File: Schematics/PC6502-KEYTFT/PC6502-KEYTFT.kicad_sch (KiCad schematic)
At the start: 47 parts, among them J1 BUS, J2 Conn_02x20_Odd_Even, J5 Conn_02x05_Odd_Even, J6 MTJ-88ARX1-FSM-LG, Q7 2N3904, Q8 2N3904, U1 W65C51NxP, U2 ATF1502AS, U21 AMS1117-3.3, U8 TXB0108PW, U9 TXB0108PW, X2 1.8432MHz

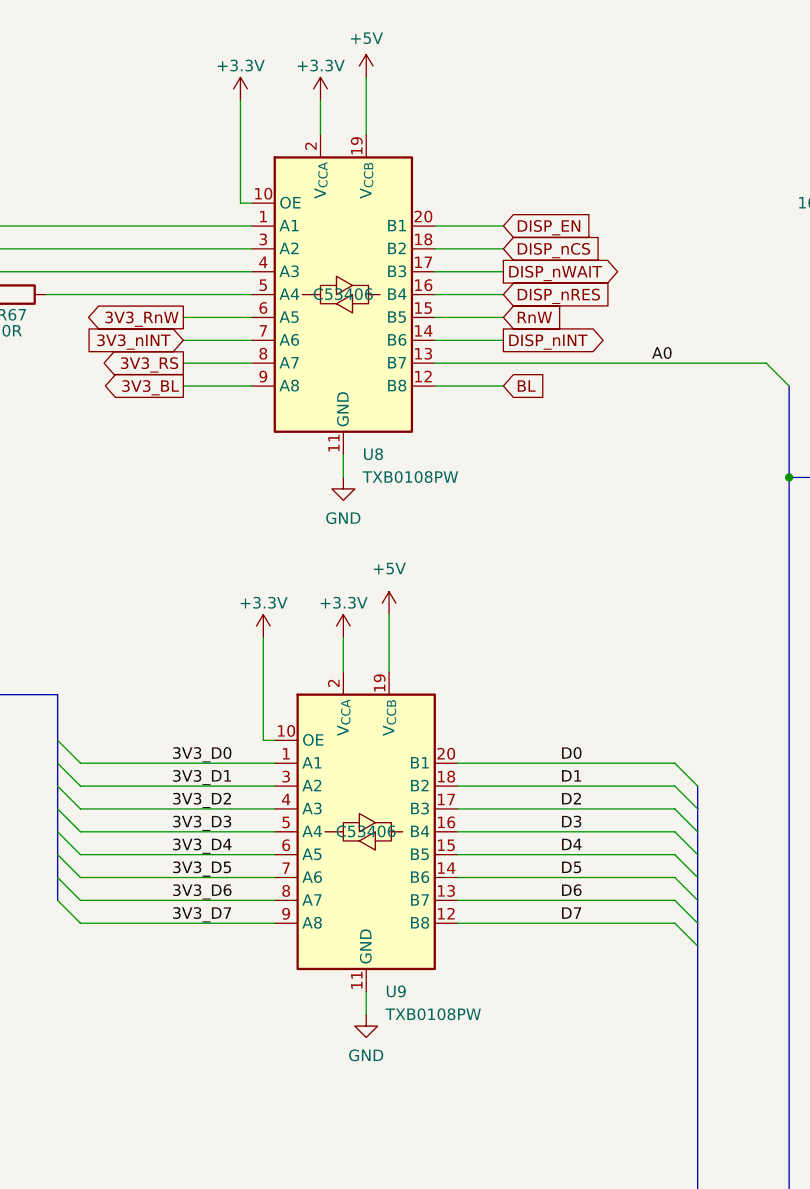
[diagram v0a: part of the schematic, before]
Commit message: Update KeyTFT CPLD
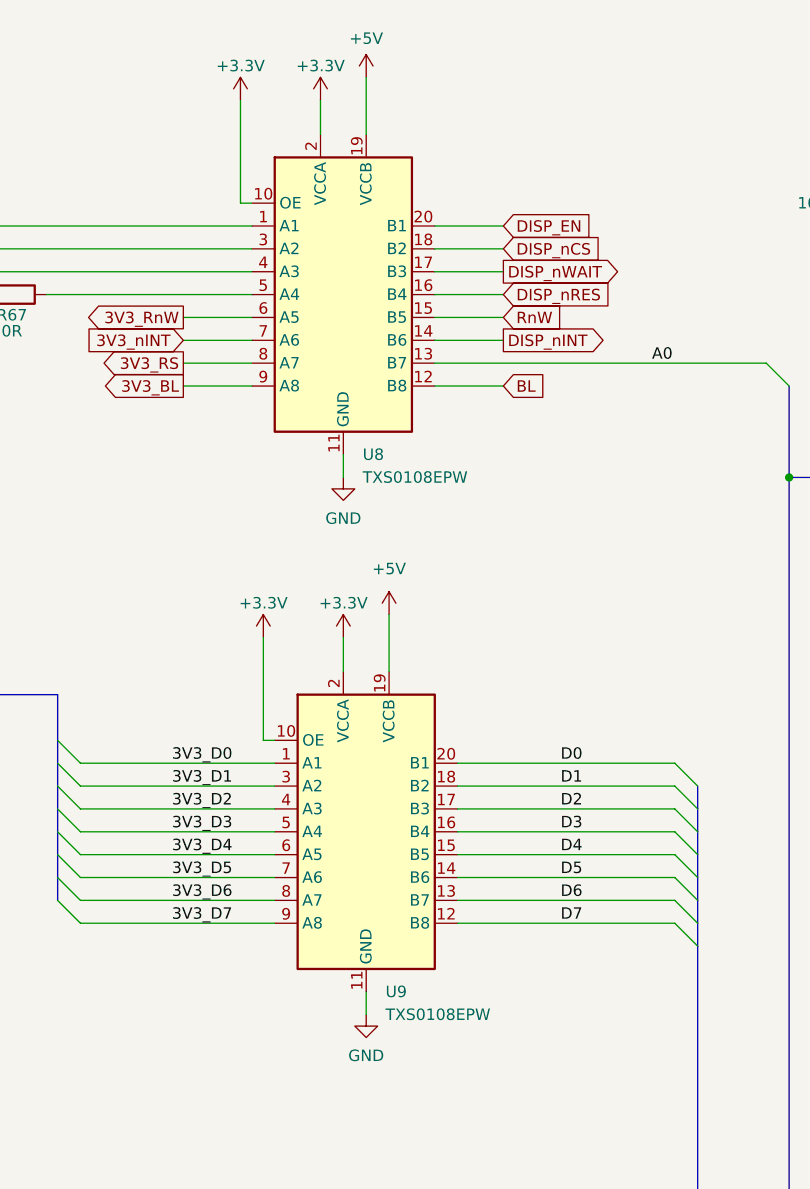
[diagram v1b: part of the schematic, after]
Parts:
- removed U8, U9: TXB0108PW, Package_SO:TSSOP-20_4.4x6.5mm_P0.65mm, symbol Logic_LevelTranslator:TXB0108PW
- added U8, U9: TXS0108EPW, Package_SO:TSSOP-20_4.4x6.5mm_P0.65mm, symbol Logic_LevelTranslator:TXS0108EPW
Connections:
- net +3.3V: now also U8.10 (OE), U8.2 (VCCA), U9.10 (OE), U9.2 (VCCA)
- net +5V: now also U8.19 (VCCB), U9.19 (VCCB)
- net 3V3_BL: now also U8.9 (A8)
- net 3V3_D0: now also U9.1 (A1)
- net 3V3_D1: now also U9.3 (A2)
- net 3V3_D2: now also U9.4 (A3)
- net 3V3_D3: now also U9.5 (A4)
- net 3V3_D4: now also U9.6 (A5)
- net 3V3_D5: now also U9.7 (A6)
- net 3V3_D6: now also U9.8 (A7)
- net 3V3_D7: now also U9.9 (A8)
- net 3V3_EN: now also U8.1 (A1)
- net 3V3_RS: now also U8.8 (A7)
- net 3V3_RnW: now also U8.6 (A5)
- net 3V3_nCS: now also U8.3 (A2)
- net 3V3_nINT: now also U8.7 (A6)
- net 3V3_nWAIT: now also U8.4 (A3)
- net A0: now also U8.13 (B7)
- net BL: now also U8.12 (B8)
- net D0: now also U9.20 (B1)
- net D1: now also U9.18 (B2)
- net D2: now also U9.17 (B3)
- net D3: now also U9.16 (B4)
- net D4: now also U9.15 (B5)
- net D5: now also U9.14 (B6)
- net D6: now also U9.13 (B7)
- net D7: now also U9.12 (B8)
- net DISP_EN: now also U8.20 (B1)
- net DISP_nCS: now also U8.18 (B2)
- net DISP_nINT: now also U8.14 (B6)
- net DISP_nRES: now also U8.16 (B4)
- net DISP_nWAIT: now also U8.17 (B3)
- net GND: now also U8.11 (GND), U9.11 (GND)
- net RnW: now also U8.15 (B5)
- net at R67.1: now also U8.5 (A4)
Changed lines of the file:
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@@
 	)
 	(symbol
+		(lib_id "Logic_LevelTranslator:TXS0108EPW")
+		(at 171.45 57.15 0)
+		(unit 1)
+		(exclude_from_sim no)
+		(in_bom yes)
+		(on_board yes)
+		(dnp no)
+		(fields_autoplaced yes)
+		(property "Reference" "U8"
+			(at 173.5933 74.93 0)
+			(effects
+				(font
+					(size 1.27 1.27)
+				)
+				(justify left)
+			)
+		)
+		(property "Value" "TXS0108EPW"
+			(at 173.5933 77.47 0)
+			(effects
+				(font
+					(size 1.27 1.27)
+				)
+				(justify left)
+			)
+		)
+		(property "Footprint" "Package_SO:TSSOP-20_4.4x6.5mm_P0.65mm"
+			(at 171.45 76.2 0)
+			(effects
+				(font
+					(size 1.27 1.27)
+				)
+				(hide yes)
+			)
+		)
+		(property "Datasheet" "www.ti.com/lit/ds/symlink/txs0108e.pdf"
+			(at 171.45 59.69 0)
+			(effects
+				(font
+					(size 1.27 1.27)
+				)
+				(hide yes)
+			)
+		)
+		(property "Description" "Bidirectional  level-shifting voltage translator, TSSOP-20"
+			(at 171.45 57.15 0)
+			(effects
+				(font
+					(size 1.27 1.27)
+				)
+				(hide yes)
+			)
+		)
+		(pin "15"
+		)
+		(pin "20"
+		)
+		(pin "2"
+		)
+		(pin "4"
+		)
+		(pin "16"
+		)
+		(pin "11"
+		)
+		(pin "13"
+		)
+		(pin "12"
+		)
+		(pin "9"
+		)
+		(pin "19"
+		)
+		(pin "18"
+		)
+		(pin "5"
+		)
+		(pin "3"
+		)
+		(pin "1"
+		)
+		(pin "10"
+		)
+		(pin "7"
+		)
+		(pin "14"
+		)
+		(pin "8"
+		)
+		(pin "17"
+		)
+		(pin "6"
+		)
+		(instances
+			(project "PC6502-KEYTFT"
+				(path "/431ed1ef-9b76-40e5-9f99-258de85faf41"
+					(reference "U8")
+					(unit 1)
+				)
+			)
+		)
+	)
+	(symbol
 		(lib_id "Connector_Generic:Conn_02x20_Odd_Even")
 		(at 92.71 67.31 0)
@@
 	)
 	(symbol
+		(lib_id "Logic_LevelTranslator:TXS0108EPW")
+		(at 173.99 116.84 0)
+		(unit 1)
+		(exclude_from_sim no)
+		(in_bom yes)
+		(on_board yes)
+		(dnp no)
+		(fields_autoplaced yes)
+		(property "Reference" "U9"
+			(at 176.1333 134.62 0)
+			(effects
+				(font
+					(size 1.27 1.27)
+				)
+				(justify left)
+			)
+		)
+		(property "Value" "TXS0108EPW"
+			(at 176.1333 137.16 0)
+			(effects
+				(font
+					(size 1.27 1.27)
+				)
+				(justify left)
+			)
+		)
+		(property "Footprint" "Package_SO:TSSOP-20_4.4x6.5mm_P0.65mm"
+			(at 173.99 135.89 0)
+			(effects
+				(font
+					(size 1.27 1.27)
+				)
+				(hide yes)
+			)
+		)
+		(property "Datasheet" "www.ti.com/lit/ds/symlink/txs0108e.pdf"
+			(at 173.99 119.38 0)
+			(effects
+				(font
+					(size 1.27 1.27)
+				)
+				(hide yes)
+			)
+		)
+		(property "Description" "Bidirectional  level-shifting voltage translator, TSSOP-20"
+			(at 173.99 116.84 0)
+			(effects
+				(font
+					(size 1.27 1.27)
+				)
+				(hide yes)
+			)
+		)
+		(pin "15"
+		)
+		(pin "20"
+		)
+		(pin "2"
+		)
+		(pin "4"
+		)
+		(pin "16"
+		)
+		(pin "11"
+		)
+		(pin "13"
+		)
+		(pin "12"
+		)
+		(pin "9"
+		)
+		(pin "19"
+		)
+		(pin "18"
+		)
+		(pin "5"
+		)
+		(pin "3"
+		)
+		(pin "1"
+		)
+		(pin "10"
+		)
+		(pin "7"
+		)
+		(pin "14"
+		)
+		(pin "8"
+		)
+		(pin "17"
+		)
+		(pin "6"
+		)
+		(instances
+			(project ""
+				(path "/431ed1ef-9b76-40e5-9f99-258de85faf41"
+					(reference "U9")
+					(unit 1)
+				)
+			)
+		)
+	)
+	(symbol
 		(lib_id "power:+5V")
 		(at 288.29 87.63 0)
@@
 	)
 	(symbol
-		(lib_id "Logic_LevelTranslator:TXB0108PW")
-		(at 173.99 116.84 0)
-		(unit 1)
-		(exclude_from_sim no)
-		(in_bom yes)
-		(on_board yes)
-		(dnp no)
-		(property "Reference" "U9"
-			(at 176.1333 134.62 0)
-			(effects
-				(font
-					(size 1.27 1.27)
-				)
-				(justify left)
-			)
-		)
-		(property "Value" "TXB0108PW"
-			(at 176.1333 137.16 0)
-			(effects
-				(font
-					(size 1.27 1.27)
-				)
-				(justify left)
-			)
-		)
-		(property "Footprint" "Package_SO:TSSOP-20_4.4x6.5mm_P0.65mm"
-			(at 173.99 135.89 0)
-			(effects
-				(font
-					(size 1.27 1.27)
-				)
-				(hide yes)
-			)
-		)
-		(property "Datasheet" "http://www.ti.com/lit/ds/symlink/txb0108.pdf"
-			(at 173.99 119.38 0)
-			(effects
-				(font
-					(size 1.27 1.27)
-				)
-				(hide yes)
-			)
-		)
-		(property "Description" "8-Bit Bidirectional Voltage-Level Translator, Auto Direction Sensing and ±15-kV ESD Protection, 1.2 - 3.6V APort, 1.65 - 5.5V BPort, TSSOP-20"
-			(at 173.99 116.84 0)
-			(effects
-				(font
-					(size 1.27 1.27)
-				)
-				(hide yes)
-			)
-		)
-		(property "LCSC" "C53406"
-			(at 173.99 116.84 0)
-			(effects
-				(font
-					(size 1.27 1.27)
-				)
-			)
-		)
-		(property "Mouser Part Number" "595-TXB0108PWR"
-			(at 173.99 116.84 0)
-			(effects
-				(font
-					(size 1.27 1.27)
-				)
-				(hide yes)
-			)
-		)
-		(pin "4"
-		)
-		(pin "16"
-		)
-		(pin "3"
-		)
-		(pin "9"
-		)
-		(pin "6"
-		)
-		(pin "1"
-		)
-		(pin "10"
-		)
-		(pin "5"
-		)
-		(pin "19"
-		)
-		(pin "8"
-		)
-		(pin "2"
-		)
-		(pin "20"
-		)
-		(pin "11"
-		)
-		(pin "7"
-		)
-		(pin "18"
-		)
-		(pin "17"
-		)
-		(pin "15"
-		)
-		(pin "14"
-		)
-		(pin "13"
-		)
-		(pin "12"
-		)
-		(instances
-			(project "PC6502-KEYTFT"
-				(path "/431ed1ef-9b76-40e5-9f99-258de85faf41"
-					(reference "U9")
-					(unit 1)
-				)
-			)
-		)
-	)
-	(symbol
 		(lib_id "power:+3.3V")
 		(at 168.91 35.56 0)
@@
 					(unit 1)
 				)
-			)
-		)
-	)
-	(symbol
-		(lib_id "Logic_LevelTranslator:TXB0108PW")
-		(at 171.45 57.15 0)
-		(unit 1)
-		(exclude_from_sim no)
-		(in_bom yes)
-		(on_board yes)
-		(dnp no)
-		(property "Reference" "U8"
-			(at 173.5933 74.93 0)
-			(effects
-				(font
-					(size 1.27 1.27)
-				)
-				(justify left)
-			)
-		)
-		(property "Value" "TXB0108PW"
-			(at 173.5933 77.47 0)
-			(effects
-				(font
-					(size 1.27 1.27)
-				)
-				(justify left)
-			)
-		)
-		(property "Footprint" "Package_SO:TSSOP-20_4.4x6.5mm_P0.65mm"
-			(at 171.45 76.2 0)
-			(effects
-				(font
-					(size 1.27 1.27)
-				)
-				(hide yes)
-			)
-		)
-		(property "Datasheet" "http://www.ti.com/lit/ds/symlink/txb0108.pdf"
-			(at 171.45 59.69 0)
-			(effects
-				(font
-					(size 1.27 1.27)
-				)
-				(hide yes)
-			)
-		)
-		(property "Description" "8-Bit Bidirectional Voltage-Level Translator, Auto Direction Sensing and ±15-kV ESD Protection, 1.2 - 3.6V APort, 1.65 - 5.5V BPort, TSSOP-20"
-			(at 171.45 57.15 0)
-			(effects
-				(font
-					(size 1.27 1.27)
-				)
-				(hide yes)
-			)
-		)
-		(property "LCSC" "C53406"
-			(at 171.45 57.15 0)
-			(effects
-				(font
-					(size 1.27 1.27)
-				)
-			)
-		)
-		(property "Mouser Part Number" "595-TXB0108PWR"
-			(at 171.45 57.15 0)
-			(effects
-				(font
-					(size 1.27 1.27)
-				)
-				(hide yes)
-			)
-		)
-		(pin "4"
-		)
-		(pin "16"
-		)
-		(pin "3"
-		)
-		(pin "9"
-		)
-		(pin "6"
-		)
-		(pin "1"
-		)
-		(pin "10"
-		)
-		(pin "5"
-		)
-		(pin "19"
-		)
-		(pin "8"
-		)
-		(pin "2"
-		)
-		(pin "20"
-		)
-		(pin "11"
-		)
-		(pin "7"
-		)
-		(pin "18"
-		)
-		(pin "17"
-		)
-		(pin "15"
-		)
-		(pin "14"
-		)
-		(pin "13"
-		)
-		(pin "12"
-		)
-		(instances
-			(project "PC6502-KEYTFT"
-				(path "/431ed1ef-9b76-40e5-9f99-258de85faf41"
-					(reference "U8")
-					(unit 1)
-				)
